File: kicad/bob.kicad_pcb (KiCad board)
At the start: 2 copper layers, 47 x 18.4 mm, 45 parts, among them J1 GPIO (Optional), J2 Mini USB Female, J3 Battery Connector, J4 GPIO (Optional), SW1 Screw Switch, U1 RP2040, U2 W25Q64JVSS, U3 NCP1117-3.3_SOT223, U4 MPU-6050, U5 BMP180, Y1 12MHz

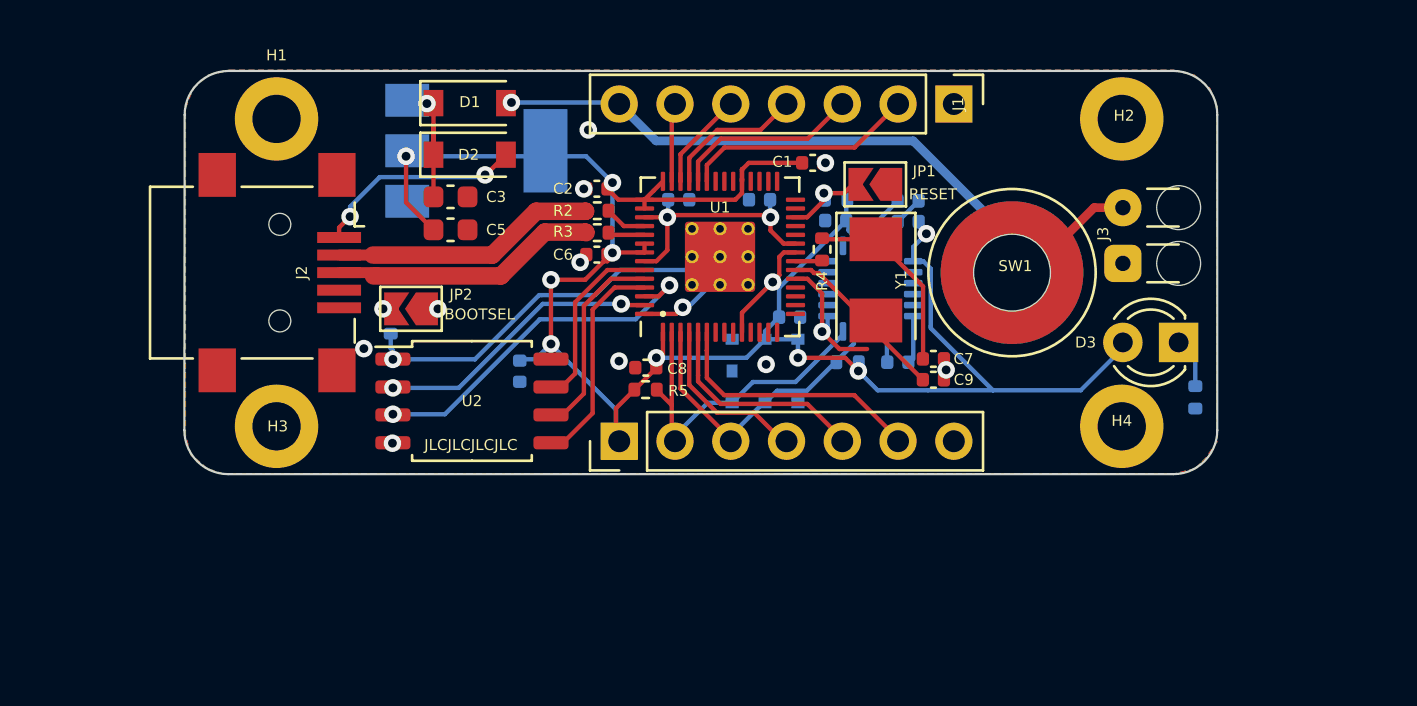
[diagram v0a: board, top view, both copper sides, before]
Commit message: Rev 3, issued for production
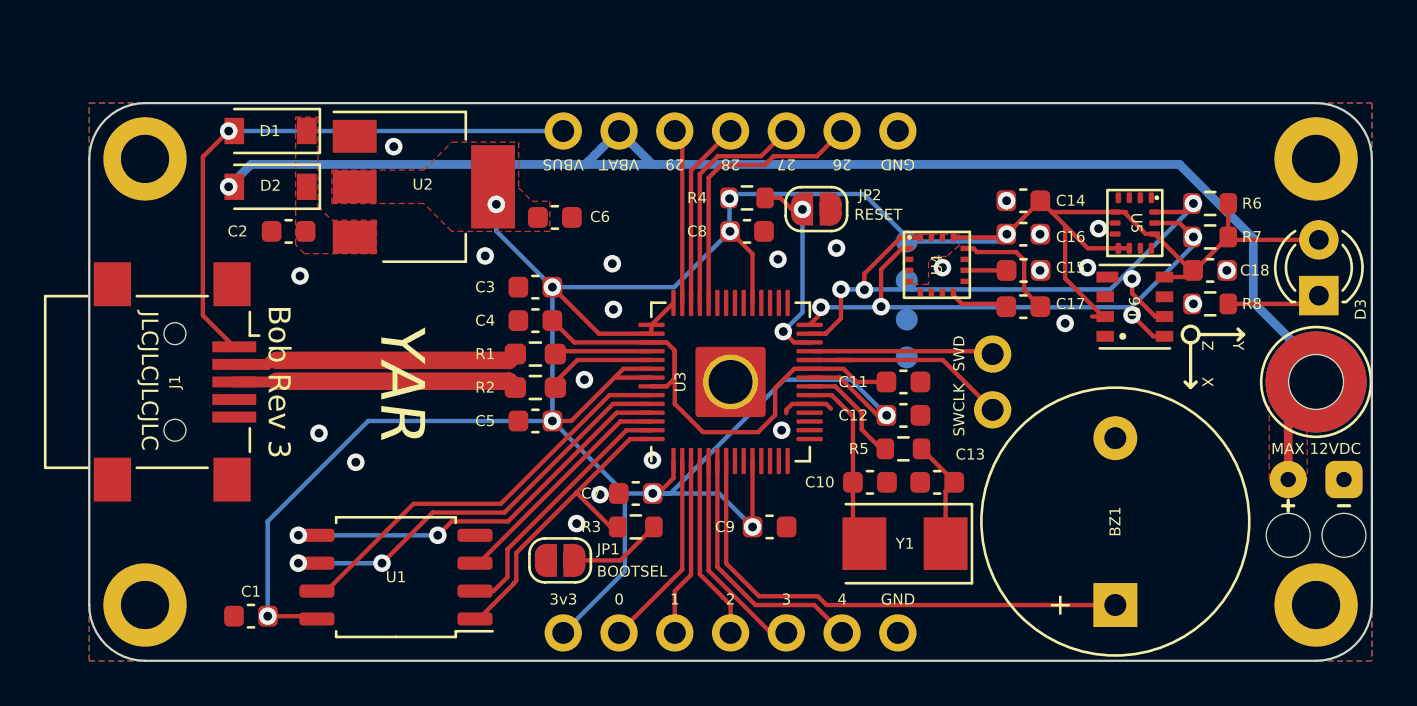
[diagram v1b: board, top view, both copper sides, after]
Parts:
- removed the YAR at (22.6, 25.5)
- added BZ1: Buzzer, Buzzer_Beeper:Buzzer_12x9.5RM7.6, F.Cu at (60.7, 40.6)
- added C17: 220n, Capacitor_SMD:C_0603_1608Metric, F.Cu at (56.5, 27.1)
- added C18: 100n, Capacitor_SMD:C_0603_1608Metric, F.Cu at (65.0, 25.4)
- added J5: Conn_01x03_Male, Connector_PinHeader_2.54mm:PinHeader_1x02_P2.54mm_Vertical, B.Cu at (55.1, 29.2)
- added TP1: TestPoint, TestPoint:TestPoint_Pad_D1.0mm, B.Cu at (51.2, 24.1)
- added TP2: TestPoint, TestPoint:TestPoint_Pad_D1.0mm, B.Cu at (51.2, 25.9)
- added TP3: TestPoint, TestPoint:TestPoint_Pad_D1.0mm, B.Cu at (51.2, 27.6)
- added TP4: TestPoint, TestPoint:TestPoint_Pad_D1.0mm, B.Cu at (51.2, 29.4)
- added U6: HP203B, RP2040_minimal:LGA-8_3.6x3.8x0.9P, F.Cu at (61.6, 27.1)
- added YAR: LOGO, Logos:YAR_Logo, F.Cu at (28.2, 30.5)
- C1, C8: footprint Capacitor_SMD:C_0402_1005Metric -> Capacitor_SMD:C_0603_1608Metric
- C10: value 100n -> 4p; footprint Capacitor_SMD:C_0402_1005Metric -> Capacitor_SMD:C_0603_1608Metric; moved to F.Cu
- C11, C12, C14, C15: footprint Capacitor_SMD:C_0402_1005Metric -> Capacitor_SMD:C_0603_1608Metric; moved to F.Cu
- C13: value 1u -> 4p; footprint Capacitor_SMD:C_0402_1005Metric -> Capacitor_SMD:C_0603_1608Metric; moved to F.Cu
- C16: value 1u -> 4.7u; footprint Capacitor_SMD:C_0402_1005Metric -> Capacitor_SMD:C_0603_1608Metric; moved to F.Cu
- C2: value 1u -> 10u; footprint Capacitor_SMD:C_0402_1005Metric -> Capacitor_SMD:C_0603_1608Metric
- C3: value 10u -> 1u
- C4: value 100n -> 1u; footprint Capacitor_SMD:C_0402_1005Metric -> Capacitor_SMD:C_0603_1608Metric; moved to F.Cu
- C5: value 10u -> 100n
- C6: value 100n -> 10u; footprint Capacitor_SMD:C_0402_1005Metric -> Capacitor_SMD:C_0603_1608Metric
- C7, C9: value 27p -> 100n; footprint Capacitor_SMD:C_0402_1005Metric -> Capacitor_SMD:C_0603_1608Metric
- J1: value GPIO (Optional) -> Mini USB Female; footprint Connector_PinHeader_2.54mm:PinHeader_1x07_P2.54mm_Vertical -> Connector_USB:USB_Mini-B_Lumberg_2486_01_Horizontal
- J2: value Mini USB Female -> GPIO (Optional); footprint Connector_USB:USB_Mini-B_Lumberg_2486_01_Horizontal -> Connector_PinHeader_2.54mm:PinHeader_1x07_P2.54mm_Vertical_NoSilk
- J3: value Battery Connector -> GPIO (Optional); footprint Connector_Wire:Compact_Relief -> Connector_PinHeader_2.54mm:PinHeader_1x07_P2.54mm_Vertical_NoSilk
- J4: value GPIO (Optional) -> Battery Connector; footprint Connector_PinHeader_2.54mm:PinHeader_1x07_P2.54mm_Vertical -> Connector_Wire:Compact_Relief; moved to B.Cu
- JP1: value RESET -> BOOTSEL; footprint Jumper:SolderJumper-2_P1.3mm_Open_TrianglePad1.0x1.5mm -> Jumper:SolderJumper-2_P1.3mm_Open_RoundedPad1.0x1.5mm
- JP2: value BOOTSEL -> RESET; footprint Jumper:SolderJumper-2_P1.3mm_Open_TrianglePad1.0x1.5mm -> Jumper:SolderJumper-2_P1.3mm_Open_RoundedPad1.0x1.5mm
- R1: value 1k -> 27; footprint Resistor_SMD:R_0402_1005Metric -> Resistor_SMD:R_0603_1608Metric_Pad0.98x0.95mm_HandSolder; moved to F.Cu
- R2: footprint Resistor_SMD:R_0402_1005Metric -> Resistor_SMD:R_0603_1608Metric_Pad0.98x0.95mm_HandSolder
- R3: value 27 -> 1k; footprint Resistor_SMD:R_0402_1005Metric -> Resistor_SMD:R_0603_1608Metric
- R4: footprint Resistor_SMD:R_0402_1005Metric -> Resistor_SMD:R_0603_1608Metric
- R5: value 4k7 -> 1k; footprint Resistor_SMD:R_0402_1005Metric -> Resistor_SMD:R_0603_1608Metric
- R6: value 1k -> 10k; footprint Resistor_SMD:R_0402_1005Metric -> Resistor_SMD:R_0603_1608Metric; moved to F.Cu
- R7: value 4k7 -> 10k; footprint Resistor_SMD:R_0402_1005Metric -> Resistor_SMD:R_0603_1608Metric; moved to F.Cu
- R8: value 1k -> 100; footprint Resistor_SMD:R_0402_1005Metric -> Resistor_SMD:R_0603_1608Metric; moved to F.Cu
- SW1: footprint Connector:Screw_Switch_M3 -> Connector:Screw_Switch_M2
- U1: value RP2040 -> W25Q64JVSS; footprint RP2040_minimal:RP2040-QFN-56 -> Package_SO:SOIC-8_5.23x5.23mm_P1.27mm
- U2: value W25Q64JVSS -> AMS1117-3.3; footprint Package_SO:SOIC-8_5.23x5.23mm_P1.27mm -> Package_TO_SOT_SMD:SOT-223-3_TabPin2
- U3: value NCP1117-3.3_SOT223 -> RP2040; footprint Package_TO_SOT_SMD:SOT-223-3_TabPin2 -> RP2040_minimal:RP2040-QFN-56_HS; moved to F.Cu
- U4: value MPU-6050 -> QMC5883L; footprint Sensor_Motion:InvenSense_QFN-24_4x4mm_P0.5mm -> Silicon-Custom:LGA-16-3X3; moved to F.Cu
- U5: value BMP180 -> QMI8658C; footprint Silicon-Custom:BMP180 -> Silicon-Custom:14LGA_2.5x3.0; moved to F.Cu
- moved H2 49.7 mm to (16.5, 40.6)
- moved H3 48.9 mm to (69.8, 20.3)
- moved R6 37.7 mm to (65.0, 22.4), turned to 0 degrees
- moved J1 37.7 mm to (17.9, 30.5)
- moved J4 33.1 mm to (71.1, 34.9), turned to 180 degrees
- moved C1 32.9 mm to (21.3, 41.1), turned to 180 degrees
- moved J3 30.5 mm to (35.6, 41.9)
- moved C15 23.8 mm to (56.5, 23.7), turned to 0 degrees
- moved JP1 22.3 mm to (35.4, 38.6), turned to 0 degrees
- moved U1 20.8 mm to (27.9, 39.4), turned to 180 degrees
- moved JP2 19.0 mm to (47.1, 22.6)
- moved U5 18.1 mm to (61.6, 23.2), turned to 90 degrees
- moved C4 17.6 mm to (34.3, 27.7)
- moved R7 17.5 mm to (65.0, 23.9)
- moved C13 17.4 mm to (52.6, 35.1)
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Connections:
- C10 pad 1: Net-(C10-Pad1) -> GND
- C10 pad 2: GND -> XIN
- C11 pad 1: +3V3 -> +1V1
- C12 pad 1: +1V1 -> +3V3
- C13 pad 1: +1V1 -> GND
- C13 pad 2: GND -> Net-(C4-Pad2)
- C16 pad 1: Net-(C16-Pad1) -> Net-(C99-Pad1)
- C2 pad 1: +3V3 -> Net-(C16-Pad1)
- C3 pad 1: Net-(D2-Pad1) -> +3V3
- C4 pad 1: +3V3 -> +1V1
- C7 pad 1: GND -> +3V3
- C7 pad 2: Net-(C7-Pad2) -> GND
- C9 pad 1: GND -> +3V3
- C9 pad 2: XIN -> GND
- D1 pad 1: Net-(D2-Pad1) -> Net-(C16-Pad1)
- D1 pad 2: +BATT -> VBUS
- D2 pad 1: Net-(D2-Pad1) -> Net-(C16-Pad1)
- D2 pad 2: VBUS -> +BATT
- J1 pad 1: GND -> VBUS
- J1 pad 2: GPIO25 -> USB_D-
- J1 pad 3: GPIO26 -> USB_D+
- J1 pad 4: GPIO27 -> unconnected-(J3-Pad4)
- J1 pad 5: GPIO28 -> GND
- J1 pad 6: GPIO29 -> GND
- J2 pad 2: USB_D- -> +BATT
- J2 pad 3: USB_D+ -> GPIO29
- J2 pad 4: unconnected-(J2-Pad4) -> GPIO28
- J2 pad 5: GND -> GPIO27
- J2 pad 6: GND -> GPIO26
- J3 pad 1: GND -> +3V3
- J3 pad 2: Net-(J3-Pad2) -> GPIO0
- J4 pad 1: +3V3 -> GND
- J4 pad 2: I2C_SDA -> Net-(J1-Pad2)
- R1 pad 1: +3V3 -> Net-(R8-Pad1)
- R1 pad 2: Net-(JP1-Pad2) -> USB_D-
- R2 pad 1: Net-(U1-Pad46) -> Net-(R7-Pad1)
- R2 pad 2: USB_D- -> USB_D+
- R3 pad 1: Net-(R3-Pad1) -> Net-(JP1-Pad2)
- R3 pad 2: USB_D+ -> QSPI_SS
- R4 pad 1: Net-(C7-Pad2) -> +3V3
- R4 pad 2: XOUT -> Net-(JP2-Pad2)
- R5 pad 1: I2C_SDA -> Net-(C4-Pad2)
- R5 pad 2: +3V3 -> XOUT
- R6 pad 1: Net-(JP2-Pad2) -> I2C_SDA
- R6 pad 2: QSPI_SS -> +3V3
- SW1 pad 1: Net-(J3-Pad2) -> Net-(J1-Pad2)
- U1 pad 1: +3V3 -> QSPI_SS
- U1 pad 2: I2C_SDA -> QSPI_SD1
- U1 pad 3: I2C_SCL -> QSPI_SD2
- U1 pad 4: GPIO2 -> GND
- U1 pad 5: GPIO3 -> QSPI_SD0
- U1 pad 6: GPIO4 -> QSPI_SCLK
- U1 pad 7: unconnected-(U1-Pad7) -> QSPI_SD3
- U1 pad 8: unconnected-(U1-Pad8) -> +3V3
- U2 pad 1: QSPI_SS -> GND
- U2 pad 2: QSPI_SD1 -> +3V3
- U2 pad 3: QSPI_SD2 -> Net-(C16-Pad1)
- U3 pad 1: GND -> +3V3
- U3 pad 2: +3V3 -> GPIO0
- U3 pad 3: Net-(D2-Pad1) -> GPIO1
- U4 pad 1: GND -> I2C_SCL
- U4 pad 10: Net-(C10-Pad1) -> Net-(C99-Pad1)
- U4 pad 12: unconnected-(U4-Pad12) -> Net-(C100-Pad2)
- U4 pad 16: unconnected-(U4-Pad16) -> I2C_SDA
- U4 pad 2: unconnected-(U4-Pad2) -> +3V3
- U4 pad 4: unconnected-(U4-Pad4) -> +3V3
- U4 pad 8: +3V3 -> Net-(C100-Pad1)
- U5 pad 1: (no net) -> GND
- U5 pad 2: +3V3 -> GND
- U5 pad 3: +3V3 -> GND
- U5 pad 4: (no net) -> unconnected-(U8-Pad4)
- U5 pad 5: I2C_SCL -> +3V3
- U5 pad 6: I2C_SDA -> GND
- Y1 pad 1: Net-(C7-Pad2) -> Net-(C4-Pad2)
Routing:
- net +3V3: track 99.6 -> 149.1 mm
- net +BATT: track 25.4 -> 59.1 mm
- net BUZZER: track 0.00 -> 23.2 mm
- net VBUS: track 9.42 -> 26.1 mm, vias 2 -> 1
- net I2C_SDA: track 16.1 -> 29.3 mm, vias 0 -> 4
- net I2C_SCL: track 14.1 -> 26.8 mm, vias 0 -> 4
- net +1V1: track 12.2 -> 23.4 mm, vias 2 -> 0
- net GPIO25: track 10.6 -> 0.00 mm
- net QSPI_SD3: track 8.37 -> 18.9 mm
- net SWCLK: track 0.00 -> 10.4 mm
- net QSPI_SCLK: track 9.17 -> 19.1 mm, vias 0 -> 2
- net GPIO0: track 0.00 -> 9.02 mm
- net Net-(JP2-Pad2): track 0.20 -> 9.22 mm, vias 1 -> 2
- net GND: track 11.0 -> 2.39 mm, vias 11 -> 22
- net Net-(C7-Pad2): track 8.45 -> 0.00 mm
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- added copper zone on F.Cu, net +3V3
- added copper zone on B.Cu, net +BATT
- added copper zone on F.Cu, net Net-(C16-Pad1)
- added copper zone on F.Cu, net Net-(J1-Pad2)
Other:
- board size 47 x 18.4 mm -> 58.4 x 25.4 mm
- board text added: "0"
- board text added: "1"
- board text added: "2"
- board text added: "26"
- board text added: "27"
- board text added: "28"
- board text added: "29"
- board text added: "3"
- board text added: "3V3"
- board text added: "3v3"
- board text added: "4"
- board text added: "Bob Rev 3"
- board text added: "GND"
- board text added: "MAX 12VDC"
- board text added: "SCL"
- board text added: "SDA"
- board text added: "SWCLK"
- board text added: "SWD"
- board text added: "Sensitive Crystal Do not route underneath"
- board text added: "USB Requires GND underneath"
- board text added: "VBAT"
- board text added: "VBUS"
- board text added: "X"
- board text added: "Y"
- board text added: "Z"
- board text removed: "Bob Rev 2"
